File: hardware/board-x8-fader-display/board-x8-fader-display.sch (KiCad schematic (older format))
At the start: 11 parts

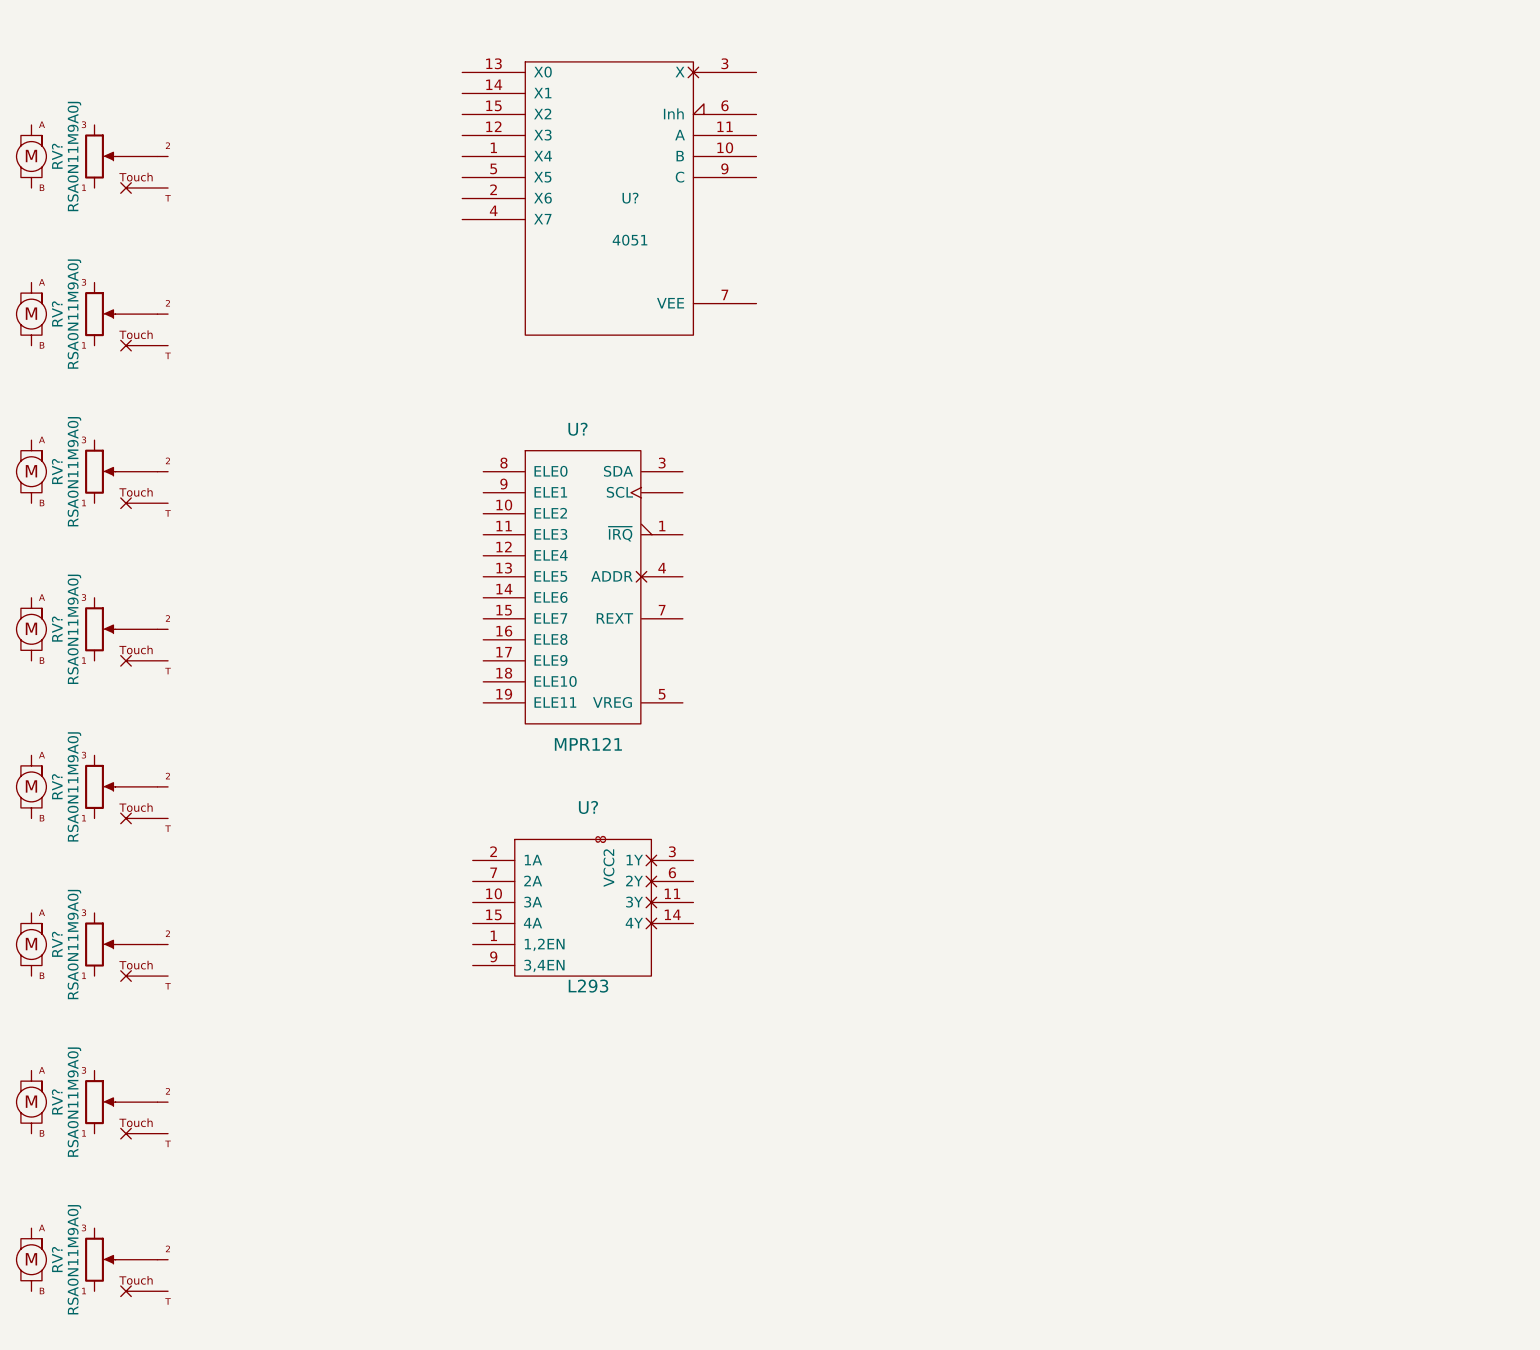
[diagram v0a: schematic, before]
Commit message: Fader board schematic updates
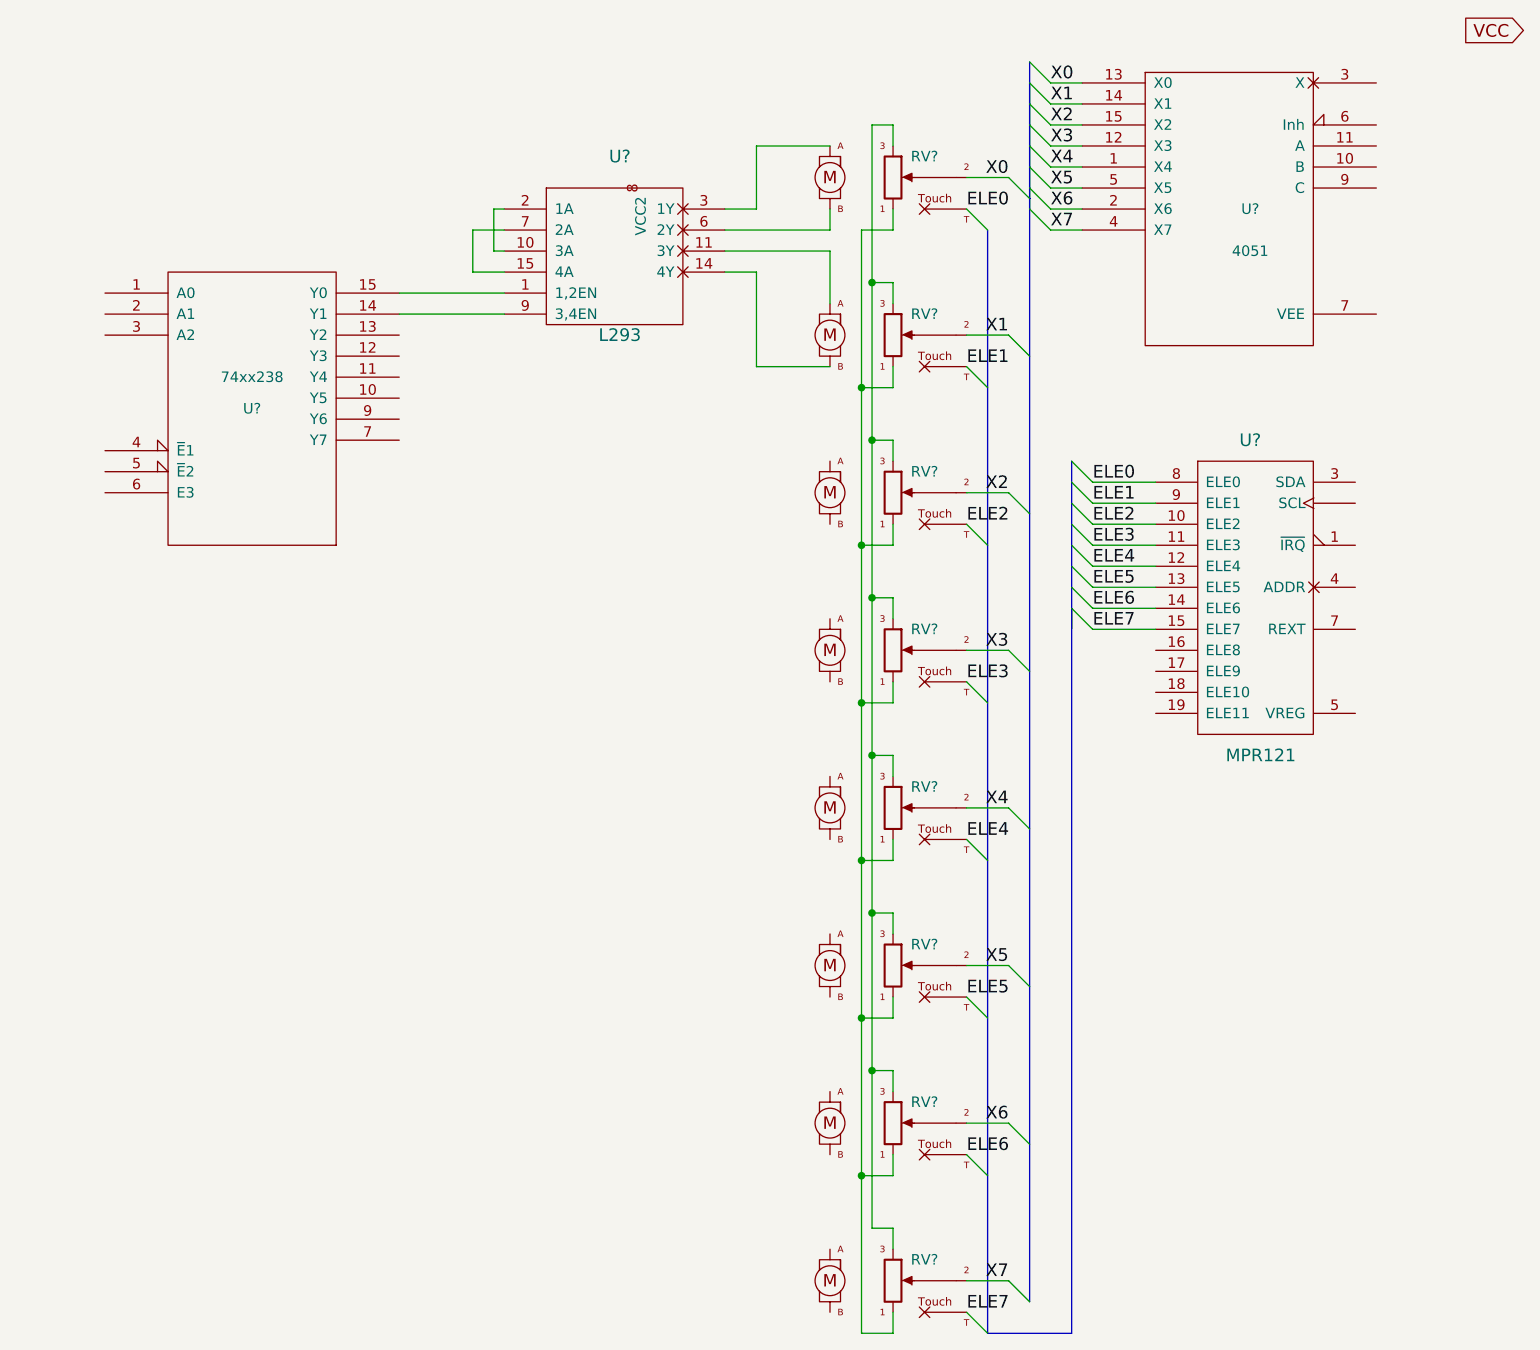
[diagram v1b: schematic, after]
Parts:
- removed U?: L293, symbol L293
- added U?: L293, symbol L293
- added U?: 74xx238, symbol 74xx238
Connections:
- net GND: now also U?.12 (GND), U?.13 (GND), U?.4 (GND), U?.5 (GND), U?.8 (GND)
- net VCC: now also U?.16 (VCC), U?.16 (VCC)
- net at RV?.1: now also RV?.1, RV?.1, RV?.1, RV?.1, RV?.1, RV?.1, RV?.1
- net X0: now reaches RV?.2
- net X0: now also U?.13 (X0)
- net at RV?.3: now also RV?.3, RV?.3, RV?.3, RV?.3, RV?.3, RV?.3, RV?.3
- net at RV?.A: now also U?.3 (1Y)
- net at RV?.B: now also U?.6 (2Y)
- net ELE0: now reaches RV?.T (Touch)
- net ELE0: now also U?.8 (ELE0)
- net X1: now reaches RV?.2
- net X1: now also U?.14 (X1)
- net at RV?.A: now also U?.11 (3Y)
- net at RV?.B: now also U?.14 (4Y)
- net ELE1: now reaches RV?.T (Touch)
- net ELE1: now also U?.9 (ELE1)
- net X2: now reaches RV?.2
- net X2: now also U?.15 (X2)
- net ELE2: now reaches RV?.T (Touch)
- net ELE2: now also U?.10 (ELE2)
- net X3: now reaches RV?.2
- net X3: now also U?.12 (X3)
- net ELE3: now reaches RV?.T (Touch)
- net ELE3: now also U?.11 (ELE3)
- net X4: now reaches RV?.2
- net X4: now also U?.1 (X4)
- net ELE4: now reaches RV?.T (Touch)
- net ELE4: now also U?.12 (ELE4)
- net X5: now reaches RV?.2
- net X5: now also U?.5 (X5)
- net ELE5: now reaches RV?.T (Touch)
- net ELE5: now also U?.13 (ELE5)
- net X6: now reaches RV?.2
- net X6: now also U?.2 (X6)
- net ELE6: now reaches RV?.T (Touch)
- net ELE6: now also U?.14 (ELE6)
- net X7: now reaches RV?.2
- net X7: now also U?.4 (X7)
- net ELE7: now reaches RV?.T (Touch)
- net ELE7: now also U?.15 (ELE7)
- new net: U?.1 (1,2EN), U?.15 (Y0)
- new net: U?.10 (3A), U?.2 (1A)
- new net: U?.15 (4A), U?.7 (2A)
- new net: U?.14 (Y1), U?.9 (3,4EN)
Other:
- moved on the sheet: RV?, U?
